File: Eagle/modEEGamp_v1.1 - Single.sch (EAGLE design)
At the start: 52 parts, among them IC2 INA217DW, P203 20k, Q202 BC557, Q204 BC557, Q206 BC547, Q208 BC547

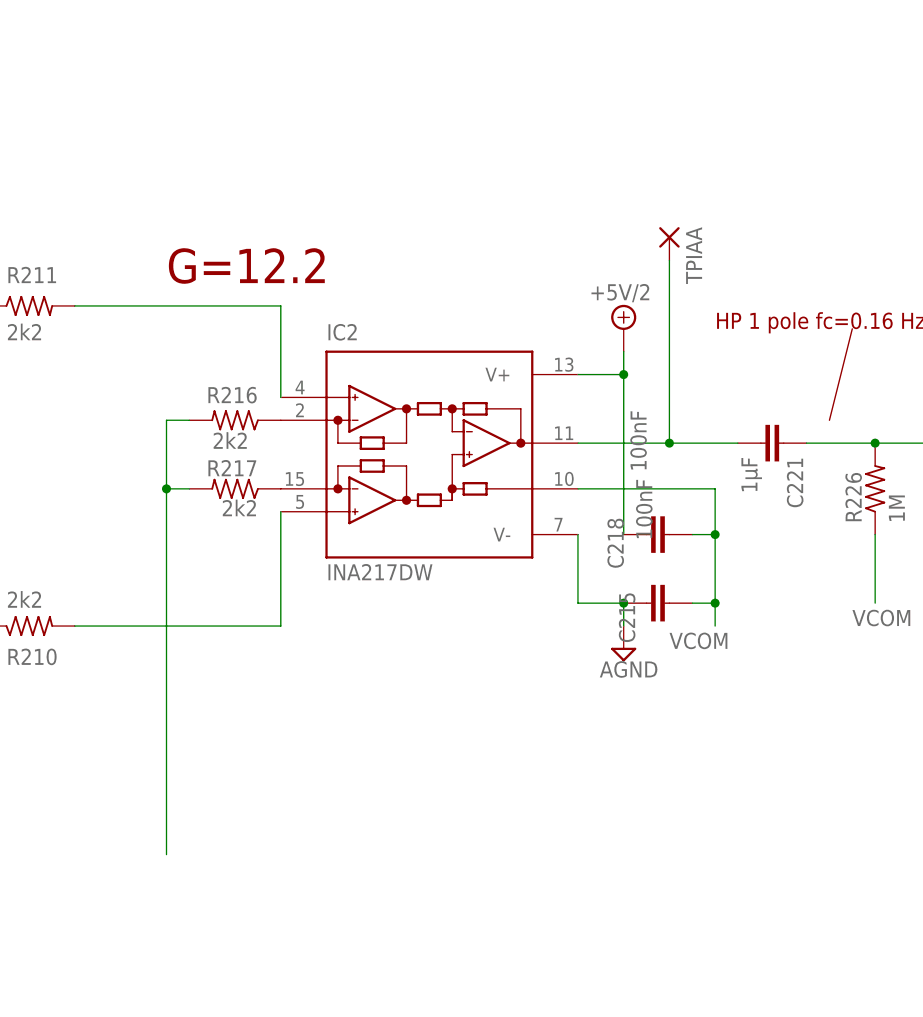
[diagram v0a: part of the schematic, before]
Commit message: Packages
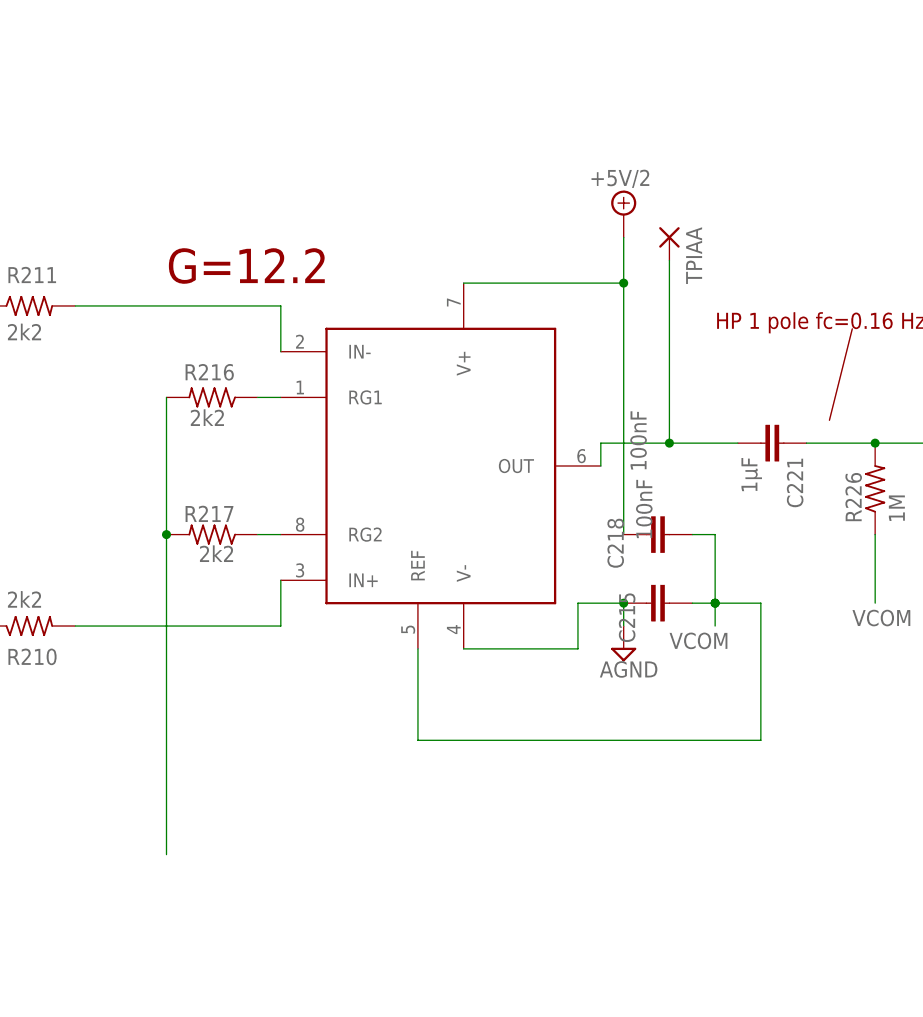
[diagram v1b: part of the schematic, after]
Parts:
- removed IC2: INA217DW, burr-brown:INA217DW
- added U$1: INA217, modEEG:INA217
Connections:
- removed net N$14: IC2.RG1, R216.1
- removed net N$20: IC2.RG2, R217.1
- new net N$1: R216.1, U$1.RG1
- new net N$2: R217.1, U$1.RG2
- net +5V/2: now also U$1.V+; no longer IC2.V+
- net AGND: now also U$1.V-; no longer IC2.V-
- net N$21: now also U$1.IN-; no longer IC2.-IN
- net N$25: now also U$1.OUT; no longer IC2.OUT
- net N$27: now also U$1.IN+; no longer IC2.+IN
- net VCOM: now also U$1.REF; no longer IC2.REF
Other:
- moved on the sheet: R216, R217
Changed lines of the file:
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@@
 <part name="R237" library="resistor" deviceset="R-US_" device="R1206" value="10k"/>
 <part name="R233" library="resistor" deviceset="R-US_" device="R1206" value="15k"/>
-<part name="IC2" library="burr-brown" deviceset="INA217" device="DW" value="INA217DW"/>
 <part name="U$2" library="EEG" deviceset="AD8021" device=""/>
 <part name="U$3" library="EEG" deviceset="AD8021" device=""/>
@@
 <part name="U$45" library="SUPPLY2" deviceset="AGND" device=""/>
 <part name="U$46" library="SUPPLY2" deviceset="AGND" device=""/>
+<part name="U$1" library="modEEG" deviceset="INA217" device=""/>
 </parts>
 <sheets>
@@
 </plain>
 <instances>
-<instance part="R216" gate="G$1" x="124.46" y="160.02" smashed="yes" rot="R180">
-<attribute name="NAME" x="121.285" y="161.925" size="1.778" layer="95"/>
-<attribute name="VALUE" x="121.92" y="156.845" size="1.778" layer="96"/>
+<instance part="R216" gate="G$1" x="121.92" y="162.56" smashed="yes" rot="R180">
+<attribute name="NAME" x="118.745" y="164.465" size="1.778" layer="95"/>
+<attribute name="VALUE" x="119.38" y="159.385" size="1.778" layer="96"/>
 </instance>
 <instance part="U$19" gate="G$1" x="167.64" y="134.62"/>
-<instance part="R217" gate="G$1" x="124.46" y="152.4" smashed="yes" rot="R180">
-<attribute name="NAME" x="127" y="155.575" size="1.778" layer="95" rot="R180"/>
-<attribute name="VALUE" x="127" y="151.13" size="1.778" layer="96" rot="R180"/>
-</instance>
-<instance part="U$26" gate="G$1" x="167.64" y="170.18"/>
+<instance part="R217" gate="G$1" x="121.92" y="147.32" smashed="yes" rot="R180">
+<attribute name="NAME" x="124.46" y="150.495" size="1.778" layer="95" rot="R180"/>
+<attribute name="VALUE" x="124.46" y="146.05" size="1.778" layer="96" rot="R180"/>
+</instance>
+<instance part="U$26" gate="G$1" x="167.64" y="182.88"/>
 <instance part="C221" gate="G$1" x="185.42" y="157.48" rot="R270"/>
 <instance part="C218" gate="G$1" x="170.18" y="147.32" smashed="yes" rot="R90">
@@
 <instance part="R237" gate="G$1" x="271.78" y="157.48"/>
 <instance part="R233" gate="G$1" x="287.02" y="157.48"/>
-<instance part="IC2" gate="G$1" x="147.32" y="157.48"/>
 <instance part="U$2" gate="IC" x="233.68" y="154.94"/>
 <instance part="U$2" gate="SUPPLY" x="259.08" y="104.14"/>
@@
 <instance part="U$45" gate="G$1" x="29.21" y="142.24"/>
 <instance part="U$46" gate="G$1" x="31.75" y="162.56"/>
+<instance part="U$1" gate="G$1" x="147.32" y="154.94"/>
 </instances>
 <busses>
@@
 <pinref part="U$19" gate="G$1" pin="AGND"/>
 <pinref part="C215" gate="G$1" pin="1"/>
-<pinref part="IC2" gate="G$1" pin="V-"/>
-<wire x1="162.56" y1="147.32" x2="162.56" y2="139.7" width="0.1524" layer="91"/>
+<pinref part="U$1" gate="G$1" pin="V-"/>
+<wire x1="149.86" y1="134.62" x2="162.56" y2="134.62" width="0.1524" layer="91"/>
+<wire x1="162.56" y1="134.62" x2="162.56" y2="139.7" width="0.1524" layer="91"/>
 </segment>
 <segment>
@@
 <net name="VCOM" class="0">
 <segment>
-<wire x1="162.56" y1="152.4" x2="177.8" y2="152.4" width="0.1524" layer="91"/>
-<wire x1="177.8" y1="152.4" x2="177.8" y2="147.32" width="0.1524" layer="91"/>
 <wire x1="177.8" y1="147.32" x2="177.8" y2="139.7" width="0.1524" layer="91"/>
 <wire x1="177.8" y1="139.7" x2="177.8" y2="137.16" width="0.1524" layer="91"/>
@@
 <wire x1="177.8" y1="139.7" x2="175.26" y2="139.7" width="0.1524" layer="91"/>
 <junction x="177.8" y="139.7"/>
-<junction x="177.8" y="147.32"/>
 <label x="172.72" y="134.62" size="1.778" layer="95"/>
 <pinref part="C218" gate="G$1" pin="2"/>
 <pinref part="C215" gate="G$1" pin="2"/>
-<pinref part="IC2" gate="G$1" pin="REF"/>
+<pinref part="U$1" gate="G$1" pin="REF"/>
+<wire x1="144.78" y1="134.62" x2="144.78" y2="124.46" width="0.1524" layer="91"/>
+<wire x1="144.78" y1="124.46" x2="182.88" y2="124.46" width="0.1524" layer="91"/>
+<wire x1="182.88" y1="124.46" x2="182.88" y2="139.7" width="0.1524" layer="91"/>
+<wire x1="182.88" y1="139.7" x2="177.8" y2="139.7" width="0.1524" layer="91"/>
+<junction x="177.8" y="139.7"/>
 </segment>
 <segment>
@@
 <net name="N$12" class="0">
 <segment>
-<wire x1="119.38" y1="160.02" x2="116.84" y2="160.02" width="0.1524" layer="91"/>
-<wire x1="116.84" y1="160.02" x2="116.84" y2="152.4" width="0.1524" layer="91"/>
-<wire x1="119.38" y1="152.4" x2="116.84" y2="152.4" width="0.1524" layer="91"/>
-<wire x1="116.84" y1="111.76" x2="116.84" y2="152.4" width="0.1524" layer="91"/>
-<junction x="116.84" y="152.4"/>
+<wire x1="116.84" y1="162.56" x2="116.84" y2="147.32" width="0.1524" layer="91"/>
+<wire x1="116.84" y1="111.76" x2="116.84" y2="147.32" width="0.1524" layer="91"/>
+<junction x="116.84" y="147.32"/>
 <pinref part="R216" gate="G$1" pin="2"/>
 <pinref part="R217" gate="G$1" pin="2"/>
@@
 <net name="+5V/2" class="0">
 <segment>
-<wire x1="167.64" y1="147.32" x2="167.64" y2="165.1" width="0.1524" layer="91"/>
+<wire x1="167.64" y1="147.32" x2="167.64" y2="175.26" width="0.1524" layer="91"/>
 <pinref part="U$26" gate="G$1" pin="+5V/2"/>
 <pinref part="C218" gate="G$1" pin="1"/>
-<pinref part="IC2" gate="G$1" pin="V+"/>
-<wire x1="167.64" y1="165.1" x2="167.64" y2="167.64" width="0.1524" layer="91"/>
-<wire x1="162.56" y1="165.1" x2="167.64" y2="165.1" width="0.1524" layer="91"/>
-<junction x="167.64" y="165.1"/>
+<wire x1="167.64" y1="175.26" x2="167.64" y2="180.34" width="0.1524" layer="91"/>
+<junction x="167.64" y="175.26"/>
+<pinref part="U$1" gate="G$1" pin="V+"/>
+<wire x1="149.86" y1="175.26" x2="167.64" y2="175.26" width="0.1524" layer="91"/>
 </segment>
 <segment>
@@
 <net name="N$25" class="0">
 <segment>
-<wire x1="162.56" y1="157.48" x2="172.72" y2="157.48" width="0.1524" layer="91"/>
+<wire x1="165.1" y1="157.48" x2="172.72" y2="157.48" width="0.1524" layer="91"/>
 <wire x1="172.72" y1="157.48" x2="180.34" y2="157.48" width="0.1524" layer="91"/>
 <wire x1="172.72" y1="177.8" x2="172.72" y2="157.48" width="0.1524" layer="91"/>
@@
 <pinref part="C221" gate="G$1" pin="2"/>
 <pinref part="TPIAA" gate="P" pin="P"/>
-<pinref part="IC2" gate="G$1" pin="OUT"/>
+<pinref part="U$1" gate="G$1" pin="OUT"/>
+<wire x1="165.1" y1="154.94" x2="165.1" y2="157.48" width="0.1524" layer="91"/>
 </segment>
 </net>
@@
 <segment>
 <wire x1="106.68" y1="172.72" x2="129.54" y2="172.72" width="0.1524" layer="91"/>
-<wire x1="129.54" y1="172.72" x2="129.54" y2="162.56" width="0.1524" layer="91"/>
+<wire x1="129.54" y1="172.72" x2="129.54" y2="167.64" width="0.1524" layer="91"/>
 <pinref part="R211" gate="G$1" pin="2"/>
-<pinref part="IC2" gate="G$1" pin="-IN"/>
+<pinref part="U$1" gate="G$1" pin="IN-"/>
 </segment>
 </net>
 <net name="N$27" class="0">
 <segment>
-<wire x1="129.54" y1="137.16" x2="129.54" y2="149.86" width="0.1524" layer="91"/>
+<wire x1="129.54" y1="137.16" x2="129.54" y2="142.24" width="0.1524" layer="91"/>
 <wire x1="106.68" y1="137.16" x2="129.54" y2="137.16" width="0.1524" layer="91"/>
 <pinref part="R210" gate="G$1" pin="2"/>
-<pinref part="IC2" gate="G$1" pin="+IN"/>
+<pinref part="U$1" gate="G$1" pin="IN+"/>
 </segment>
 </net>
@@
 </segment>
 </net>
-<net name="N$14" class="0">
-<segment>
-<pinref part="R216" gate="G$1" pin="1"/>
-<pinref part="IC2" gate="G$1" pin="RG1"/>
-</segment>
-</net>
-<net name="N$20" class="0">
-<segment>
-<pinref part="R217" gate="G$1" pin="1"/>
-<pinref part="IC2" gate="G$1" pin="RG2"/>
-</segment>
-</net>
 <net name="N$5" class="0">
 <segment>
@@
 </segment>
 </net>
+<net name="N$1" class="0">
+<segment>
+<pinref part="U$1" gate="G$1" pin="RG1"/>
+<pinref part="R216" gate="G$1" pin="1"/>
+<wire x1="127" y1="162.56" x2="129.54" y2="162.56" width="0.1524" layer="91"/>
+</segment>
+</net>
+<net name="N$2" class="0">
+<segment>
+<pinref part="U$1" gate="G$1" pin="RG2"/>
+<pinref part="R217" gate="G$1" pin="1"/>
+<wire x1="127" y1="147.32" x2="129.54" y2="147.32" width="0.1524" layer="91"/>
+</segment>
+</net>
